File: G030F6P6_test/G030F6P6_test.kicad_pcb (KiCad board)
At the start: 2 copper layers, 30 parts, among them J1 Conn_01x10_Female, J2 Conn_01x02_Male, J3 Conn_01x10_Female, J4 USB_C_Receptacle_USB2.0, J5 Conn_01x05_Female, SW1 SW_Push_SPDT, U1 CH343P, U2 STM32G030FxP, U3 XC6206P332MR

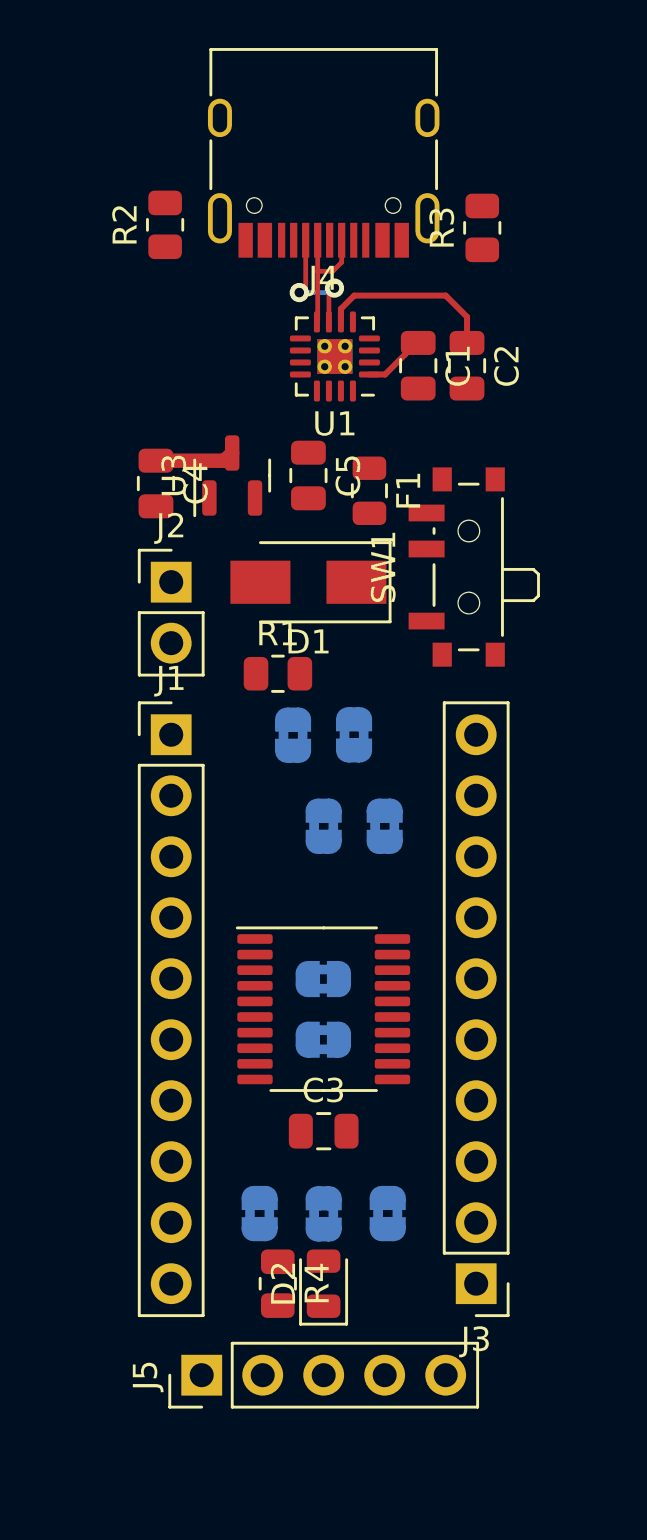
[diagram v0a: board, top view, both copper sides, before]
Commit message: 布局完成
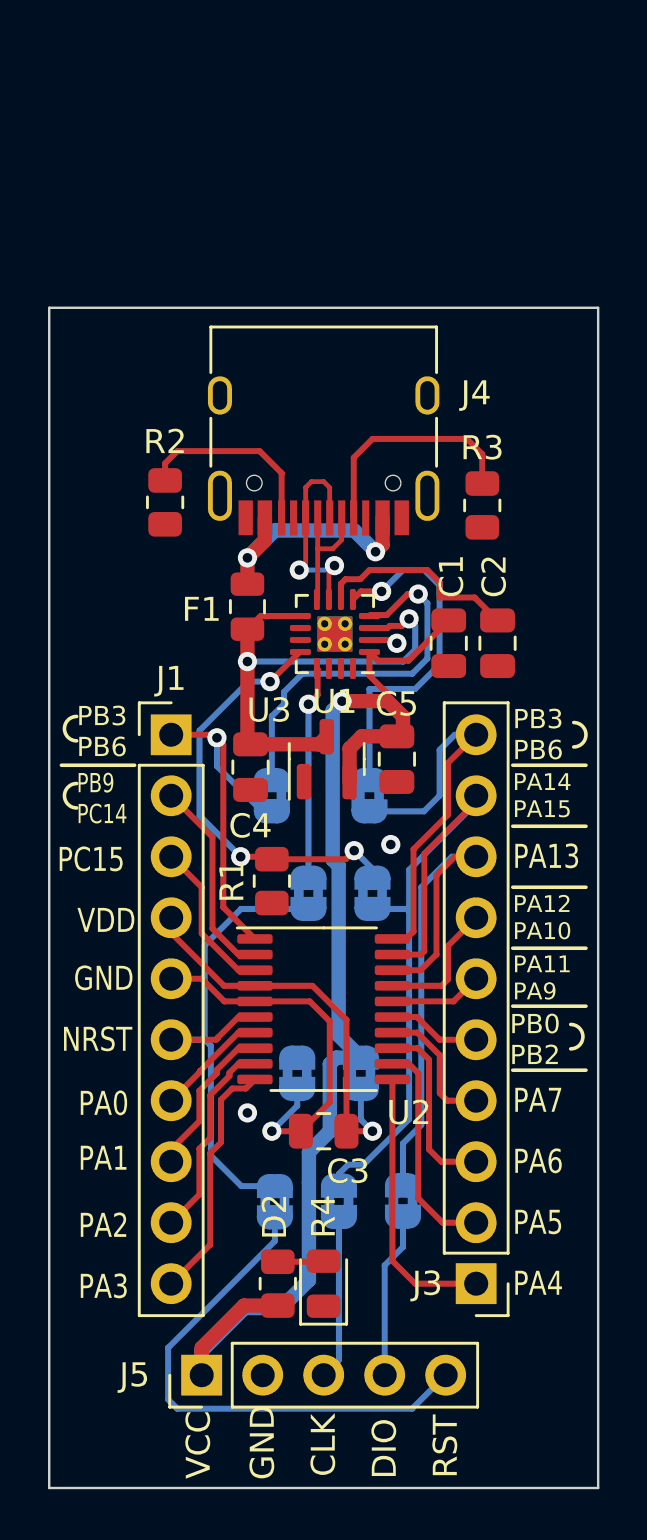
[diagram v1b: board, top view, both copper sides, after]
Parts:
- removed D1: D_Schottky, Diode_SMD:D_SMA
- removed J2: Conn_01x02_Male, Connector_PinHeader_2.54mm:PinHeader_1x02_P2.54mm_Vertical
- removed SW1: SW_Push_SPDT, Button_Switch_SMD:SW_SPDT_PCM12
- moved U3 12.4 mm to (130.9, 74.7)
- moved C4 12.4 mm to (127.8, 75.0)
- moved C5 12.4 mm to (133.9, 74.7)
- moved C2 11.6 mm to (138.0, 69.8)
- moved C1 11.6 mm to (136.0, 69.8)
- moved J4 11.6 mm to (130.8, 60.6)
- moved R3 11.6 mm to (137.4, 64.1)
- moved U1 11.6 mm to (131.3, 69.5)
- moved R2 11.6 mm to (124.2, 64.0)
- moved R1 8.64 mm to (128.7, 79.8), turned to 90 degrees
- moved JP4 7.37 mm to (132.8, 80.3)
- moved F1 7.01 mm to (127.6, 68.3)
- moved JP3 6.87 mm to (130.2, 80.3)
- moved JP7 5.99 mm to (134.1, 93.1)
- moved JP9 4.72 mm to (128.8, 93.1)
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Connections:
- C4 pad 1: +5V -> VBUS
- J5 pad 3: /SWDIO -> /SWCLK
- J5 pad 4: /SWCLK -> /SWDIO
- U1 pad 3: +5V -> VBUS
- U3 pad 3: +5V -> VBUS
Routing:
- net +3V3: track 2.58 -> 52.0 mm, vias 0 -> 1
- net /PIN19: track 0.00 -> 29.3 mm
- net /PIN18: track 0.00 -> 22.9 mm
- net /PIN6: track 0.00 -> 22.3 mm
- net /NRST: track 0.00 -> 21.7 mm
- net VBUS: track 0.00 -> 21.0 mm, vias 0 -> 2
- net /BOOT0: track 0.00 -> 17.9 mm, vias 0 -> 3
- net /PIN20: track 0.00 -> 17.2 mm
- net /PIN4: track 0.00 -> 17.1 mm, vias 0 -> 1
- net /PIN5: track 0.00 -> 15.8 mm, vias 0 -> 1
- net /TXD: track 0.00 -> 15.7 mm, vias 0 -> 1
- net /PIN1: track 0.00 -> 15.2 mm, vias 0 -> 1
- net /RXD: track 0.00 -> 14.8 mm, vias 0 -> 1
- net /PIN11: track 0.00 -> 11.4 mm
- net Net-(F1-Pad1): track 0.00 -> 10.8 mm, vias 0 -> 2
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- added copper zone on B.Cu, net GND
- added copper zone on F.Cu, net GND
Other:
- board outline added: 22.9 x 49.1 mm
- board text added: "BOT"
- board text added: "CLK"
- board text added: "DIO"
- board text added: "GND"
- board text added: "NRST"
- board text added: "PA0"
- board text added: "PA1"
- board text added: "PA11 PA9"
- board text added: "PA12 PA10"
- board text added: "PA13"
- board text added: "PA14 PA15"
- board text added: "PA2"
- board text added: "PA3"
- board text added: "PA4"
- board text added: "PA5"
- board text added: "PA6"
- board text added: "PA7"
- board text added: "PA8"
- board text added: "PB0 PB2"
- board text added: "PB3 PB6"
- board text added: "PB9 PC14"
- board text added: "PC15"
- board text added: "RST"
- board text added: "RXD"
- board text added: "STM32G030F6P6"
- board text added: "TXD"
- board text added: "VCC"
- board text added: "VDD"
- board text added: "~{RTS}"
